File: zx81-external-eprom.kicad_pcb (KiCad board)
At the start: 2 copper layers, 60.3 x 50 mm, 11 parts, among them J1 Connector ZX81, Q1 BC549, SW1 SW_DIP_x03, U1 W27C512, U2 74LS138

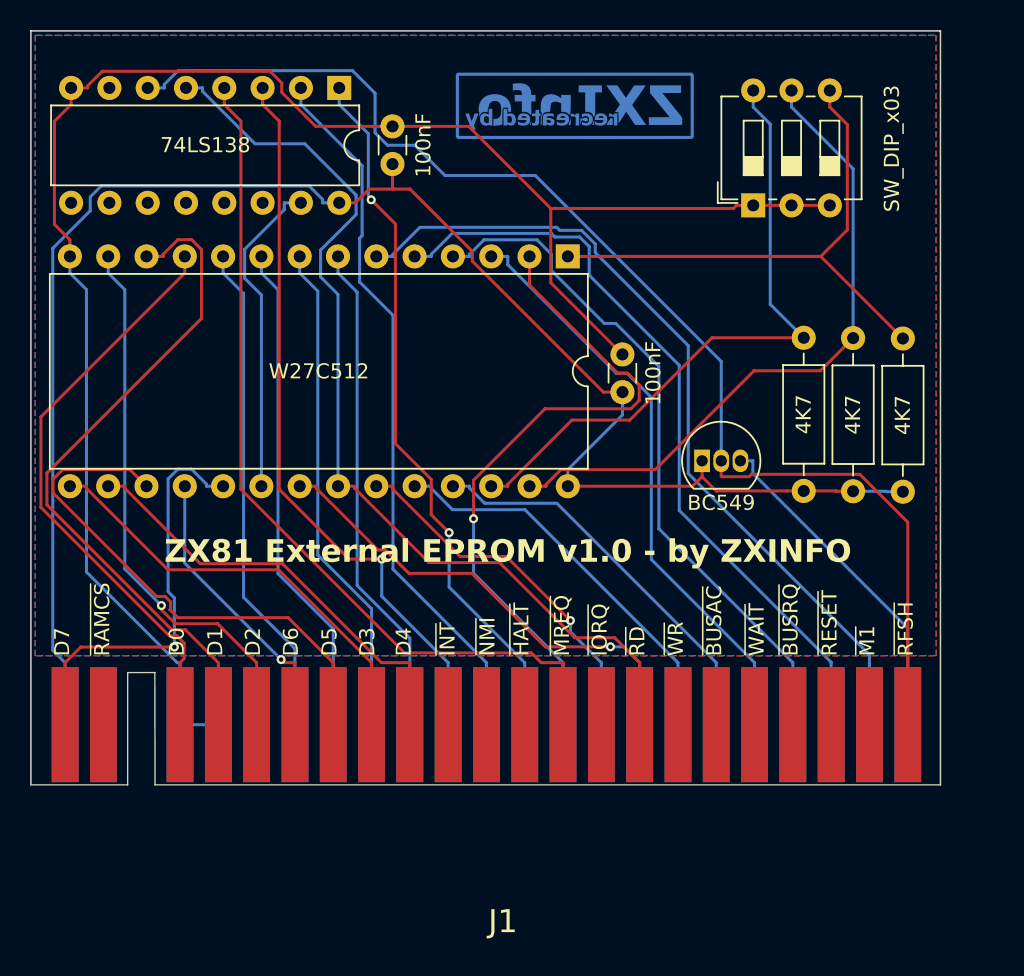
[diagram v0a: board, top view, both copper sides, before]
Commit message: small design fixes
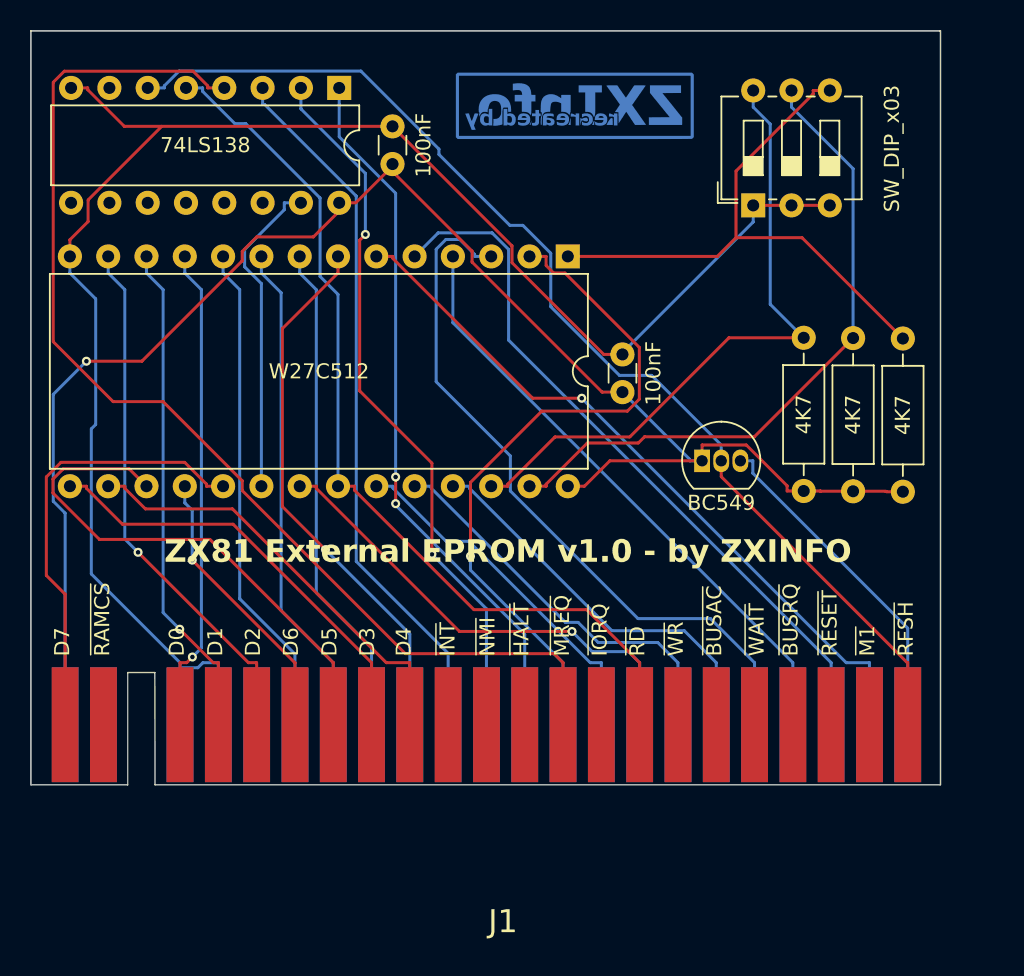
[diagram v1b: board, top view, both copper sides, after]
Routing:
- net Net-(J1-~{MREQ}): track 57.3 -> 76.5 mm
- net D1: track 45.5 -> 33.2 mm, vias 0 -> 1
- net A7: track 39.4 -> 47.6 mm
- net Net-(J1-~{RFSH}): track 83.0 -> 74.8 mm
- net A4: track 55.3 -> 48.1 mm, vias 0 -> 1
- net D0: track 39.3 -> 32.4 mm, vias 0 -> 1
- net +5V: track 112.3 -> 106.7 mm, vias 0 -> 1
- net A6: track 45.7 -> 40.4 mm
- net Net-(J1-~{RD}): track 64.2 -> 60.8 mm
- net A5: track 51.0 -> 47.7 mm
- net A3: track 33.0 -> 36.1 mm, vias 0 -> 1
- net D7: track 27.6 -> 29.8 mm, vias 1 -> 0
- net Net-(U1-A15): track 36.7 -> 38.5 mm
- net D2: track 36.8 -> 35.5 mm
- net A15: track 48.6 -> 47.4 mm, vias 1 -> 0
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- removed copper zone on B.Cu, net GND
- removed copper zone on F.Cu, net GND
